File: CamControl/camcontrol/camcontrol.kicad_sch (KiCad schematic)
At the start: 75 parts, among them J2 USB_B_Micro, J3 Conn_01x03, J5 Conn_01x02, J6 Conn_01x02, J7 Conn_01x03, J8 Conn_01x04, Q2 AO3401A, Q3 AO3401A, U1 E22-900MM22S, U2 TPS1HC30BQPWPRQ1, U3 TPS63060DSCR, U4 XC6206P332MR, U5 W25Q128JVS, U6 RP2040, U7 TPS1HC30BQPWPRQ1, X1 SX1M12.000M10F30TNN

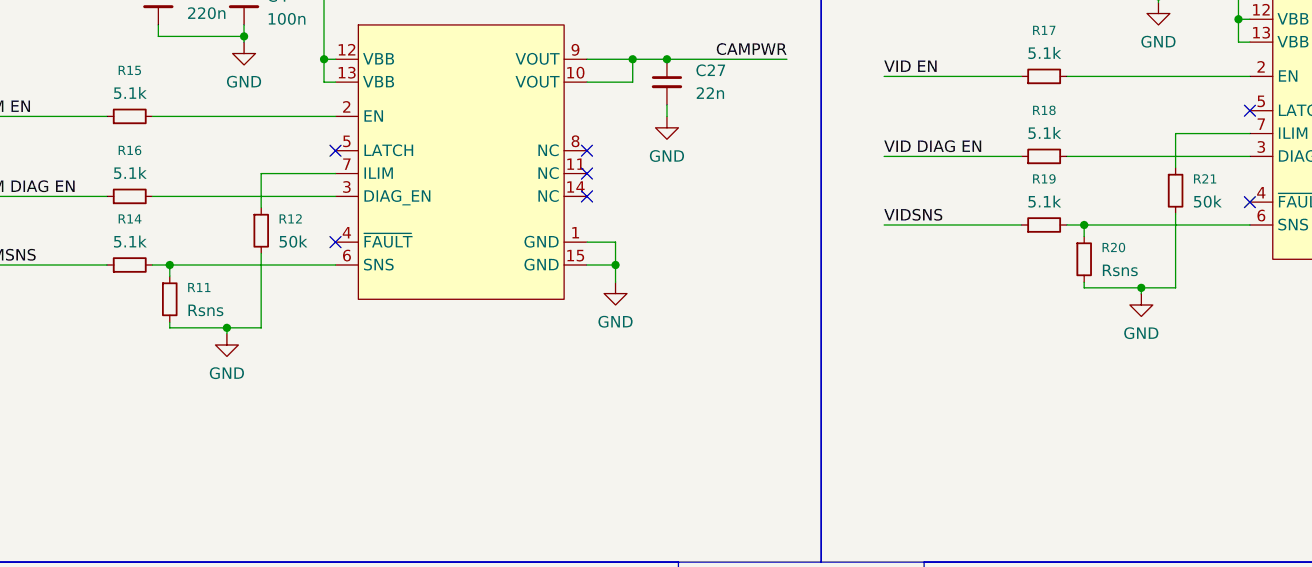
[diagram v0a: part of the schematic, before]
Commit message: cam control work and start on gruond station
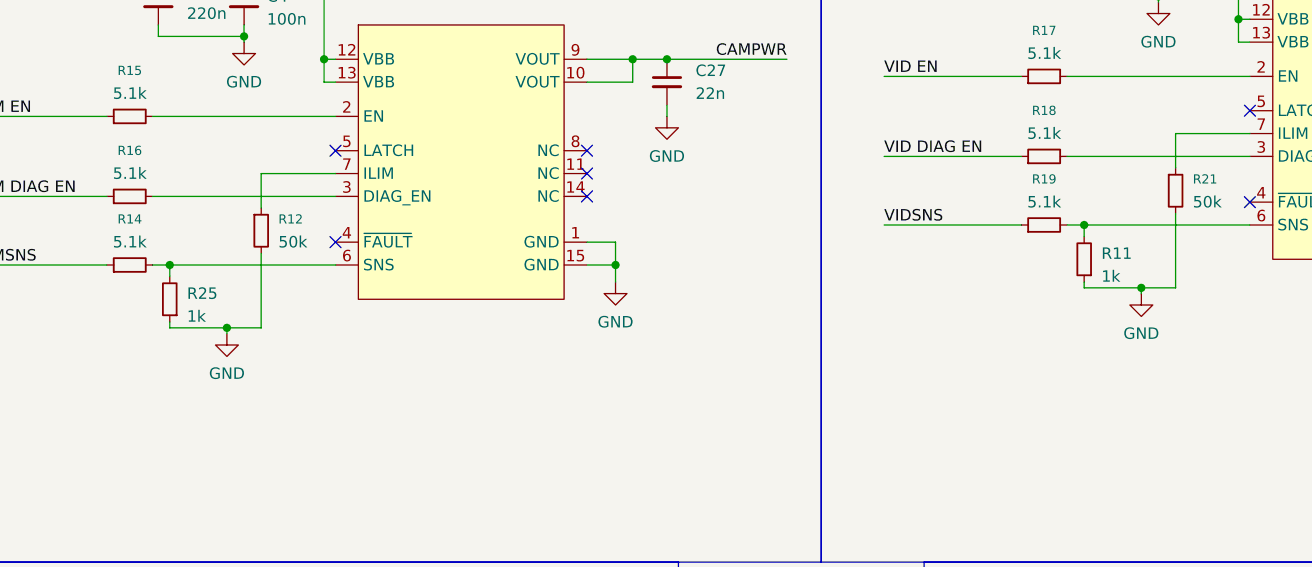
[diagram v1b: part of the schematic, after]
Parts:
- removed R20: Rsns, Resistor_SMD:R_0402_1005Metric, symbol Device:R_Small
- added R25: 1k, Resistor_SMD:R_0402_1005Metric, symbol Device:R_Small
- C26, C28: LCSC Part C1525 -> C16772
- C27, C30: LCSC Part C1525 -> C1532
- J3, J7, J8: now left out of the parts list
- R11: value Rsns -> 1k; LCSC Part (none) -> C11702
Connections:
- net GND: now also R11.1, R25.1; no longer R11.2
- net at R19.2, U7.6 (SNS): now also R11.2
- net at R14.2, U2.6 (SNS): now also R25.2; no longer R11.1
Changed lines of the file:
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@@
 			)
 		)
-		(property "LCSC Part" "C1525"
+		(property "LCSC Part" "C16772"
 			(at 244.475 33.655 0)
 			(effects
@@
 			)
 		)
-		(property "LCSC Part" "C1525"
+		(property "LCSC Part" "C16772"
 			(at 142.875 38.1 0)
 			(effects
@@
 	(symbol
 		(lib_id "Device:R_Small")
-		(at 245.745 66.675 0)
-		(unit 1)
-		(exclude_from_sim no)
-		(in_bom yes)
-		(on_board yes)
-		(dnp no)
-		(fields_autoplaced yes)
-		(property "Reference" "R20"
-			(at 247.65 65.4049 0)
-			(effects
-				(font
-					(size 1.016 1.016)
-				)
-				(justify left)
-			)
-		)
-		(property "Value" "Rsns"
-			(at 247.65 67.9449 0)
-			(effects
-				(font
-					(size 1.27 1.27)
-				)
-				(justify left)
-			)
-		)
-		(property "Footprint" "Resistor_SMD:R_0402_1005Metric"
-			(at 245.745 66.675 0)
-			(effects
-				(font
-					(size 1.27 1.27)
-				)
-				(hide yes)
-			)
-		)
-		(property "Datasheet" "~"
-			(at 245.745 66.675 0)
-			(effects
-				(font
-					(size 1.27 1.27)
-				)
-				(hide yes)
-			)
-		)
-		(property "Description" "Resistor, small symbol"
-			(at 245.745 66.675 0)
-			(effects
-				(font
-					(size 1.27 1.27)
-				)
-				(hide yes)
-			)
-		)
-		(pin "2"
-		)
-		(pin "1"
-		)
-		(instances
-			(project "camcontrol"
-				(path "/299d0a04-aa0f-4714-a339-a062da4333a5"
-					(reference "R20")
-					(unit 1)
-				)
-			)
-		)
-	)
-	(symbol
-		(lib_id "Device:R_Small")
 		(at 241.3 55.245 90)
 		(unit 1)
@@
 		(unit 1)
 		(exclude_from_sim no)
-		(in_bom yes)
+		(in_bom no)
 		(on_board yes)
 		(dnp no)
@@
 	)
 	(symbol
+		(lib_id "Device:R_Small")
+		(at 144.145 71.12 180)
+		(unit 1)
+		(exclude_from_sim no)
+		(in_bom yes)
+		(on_board yes)
+		(dnp no)
+		(fields_autoplaced yes)
+		(property "Reference" "R25"
+			(at 146.05 70.485 0)
+			(effects
+				(font
+					(size 1.27 1.27)
+				)
+				(justify right)
+			)
+		)
+		(property "Value" "1k"
+			(at 146.05 73.025 0)
+			(effects
+				(font
+					(size 1.27 1.27)
+				)
+				(justify right)
+			)
+		)
+		(property "Footprint" "Resistor_SMD:R_0402_1005Metric"
+			(at 144.145 71.12 0)
+			(effects
+				(font
+					(size 1.27 1.27)
+				)
+				(hide yes)
+			)
+		)
+		(property "Datasheet" "~"
+			(at 144.145 71.12 0)
+			(effects
+				(font
+					(size 1.27 1.27)
+				)
+				(hide yes)
+			)
+		)
+		(property "Description" "Resistor, small symbol"
+			(at 144.145 71.12 0)
+			(effects
+				(font
+					(size 1.27 1.27)
+				)
+				(hide yes)
+			)
+		)
+		(property "LCSC Part" "C11702"
+			(at 144.145 71.12 0)
+			(effects
+				(font
+					(size 1.27 1.27)
+				)
+				(hide yes)
+			)
+		)
+		(property "LCSC_Part" ""
+			(at 144.145 71.12 0)
+			(effects
+				(font
+					(size 1.27 1.27)
+				)
+				(hide yes)
+			)
+		)
+		(pin "1"
+		)
+		(pin "2"
+		)
+		(instances
+			(project "camcontrol"
+				(path "/299d0a04-aa0f-4714-a339-a062da4333a5"
+					(reference "R25")
+					(unit 1)
+				)
+			)
+		)
+	)
+	(symbol
 		(lib_id "power:GND")
 		(at 250.825 214.63 0)
@@
 		(unit 1)
 		(exclude_from_sim no)
-		(in_bom yes)
+		(in_bom no)
 		(on_board yes)
 		(dnp no)
@@
 			)
 		)
-		(property "LCSC Part" "C1525"
+		(property "LCSC Part" "C1532"
 			(at 199.39 46.99 0)
 			(effects
@@
 			)
 		)
-		(property "LCSC Part" "C1525"
+		(property "LCSC Part" "C1532"
 			(at 300.99 42.545 0)
 			(effects
@@
 	)
 	(symbol
-		(lib_id "Device:R_Small")
-		(at 144.145 71.12 0)
-		(unit 1)
-		(exclude_from_sim no)
-		(in_bom yes)
-		(on_board yes)
-		(dnp no)
-		(fields_autoplaced yes)
-		(property "Reference" "R11"
-			(at 146.05 69.8499 0)
-			(effects
-				(font
-					(size 1.016 1.016)
-				)
-				(justify left)
-			)
-		)
-		(property "Value" "Rsns"
-			(at 146.05 72.3899 0)
-			(effects
-				(font
-					(size 1.27 1.27)
-				)
-				(justify left)
-			)
-		)
-		(property "Footprint" "Resistor_SMD:R_0402_1005Metric"
-			(at 144.145 71.12 0)
-			(effects
-				(font
-					(size 1.27 1.27)
-				)
-				(hide yes)
-			)
-		)
-		(property "Datasheet" "~"
-			(at 144.145 71.12 0)
-			(effects
-				(font
-					(size 1.27 1.27)
-				)
-				(hide yes)
-			)
-		)
-		(property "Description" "Resistor, small symbol"
-			(at 144.145 71.12 0)
-			(effects
-				(font
-					(size 1.27 1.27)
-				)
-				(hide yes)
-			)
-		)
-		(pin "2"
-		)
-		(pin "1"
-		)
-		(instances
-			(project ""
-				(path "/299d0a04-aa0f-4714-a339-a062da4333a5"
-					(reference "R11")
-					(unit 1)
-				)
-			)
-		)
-	)
-	(symbol
 		(lib_id "power:+3V3")
 		(at 74.295 170.815 0)
@@
 		(unit 1)
 		(exclude_from_sim no)
-		(in_bom yes)
+		(in_bom no)
 		(on_board yes)
 		(dnp no)
@@
 					(unit 1)
 				)
+			)
+		)
+	)
+	(symbol
+		(lib_id "Device:R_Small")
+		(at 245.745 66.675 180)
+		(unit 1)
+		(exclude_from_sim no)
+		(in_bom yes)
+		(on_board yes)
+		(dnp no)
+		(fields_autoplaced yes)
+		(property "Reference" "R11"
+			(at 247.65 66.04 0)
+			(effects
+				(font
+					(size 1.27 1.27)
+				)
+				(justify right)
+			)
+		)
+		(property "Value" "1k"
+			(at 247.65 68.58 0)
+			(effects
+				(font
+					(size 1.27 1.27)
+				)
+				(justify right)
+			)
+		)
+		(property "Footprint" "Resistor_SMD:R_0402_1005Metric"
+			(at 245.745 66.675 0)
+			(effects
+				(font
+					(size 1.27 1.27)
+				)
+				(hide yes)
+			)
+		)
+		(property "Datasheet" "~"
+			(at 245.745 66.675 0)
+			(effects
+				(font
+					(size 1.27 1.27)
+				)
+				(hide yes)
+			)
+		)
+		(property "Description" "Resistor, small symbol"
+			(at 245.745 66.675 0)
+			(effects
+				(font
+					(size 1.27 1.27)
+				)
+				(hide yes)
+			)
+		)
+		(property "LCSC Part" "C11702"
+			(at 245.745 66.675 0)
+			(effects
+				(font
+					(size 1.27 1.27)
+				)
+				(hide yes)
+			)
+		)
+		(property "LCSC_Part" ""
+			(at 245.745 66.675 0)
+			(effects
+				(font
+					(size 1.27 1.27)
+				)
+				(hide yes)
+			)
+		)
+		(pin "1"
+		)
+		(pin "2"
+		)
+		(instances
+			(project "camcontrol"
+				(path "/299d0a04-aa0f-4714-a339-a062da4333a5"
+					(reference "R11")
+					(unit 1)
+				)
